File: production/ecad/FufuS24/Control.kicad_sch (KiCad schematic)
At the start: 28 parts, among them IC1 NLVPCA9535EDTR2G, J2 Conn_01x02, U1 RP2040, U2 W25Q128JVS

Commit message: efan 5
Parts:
- J2: footprint (none) -> footprints:CON_5025840270_MOL
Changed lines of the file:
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@@
       (effects (font (size 1.27 1.27)))
     )
-    (property "Footprint" "" (at 20.955 85.09 0)
+    (property "Footprint" "footprints:CON_5025840270_MOL" (at 20.955 85.09 0)
       (effects (font (size 1.27 1.27)) hide)
     )

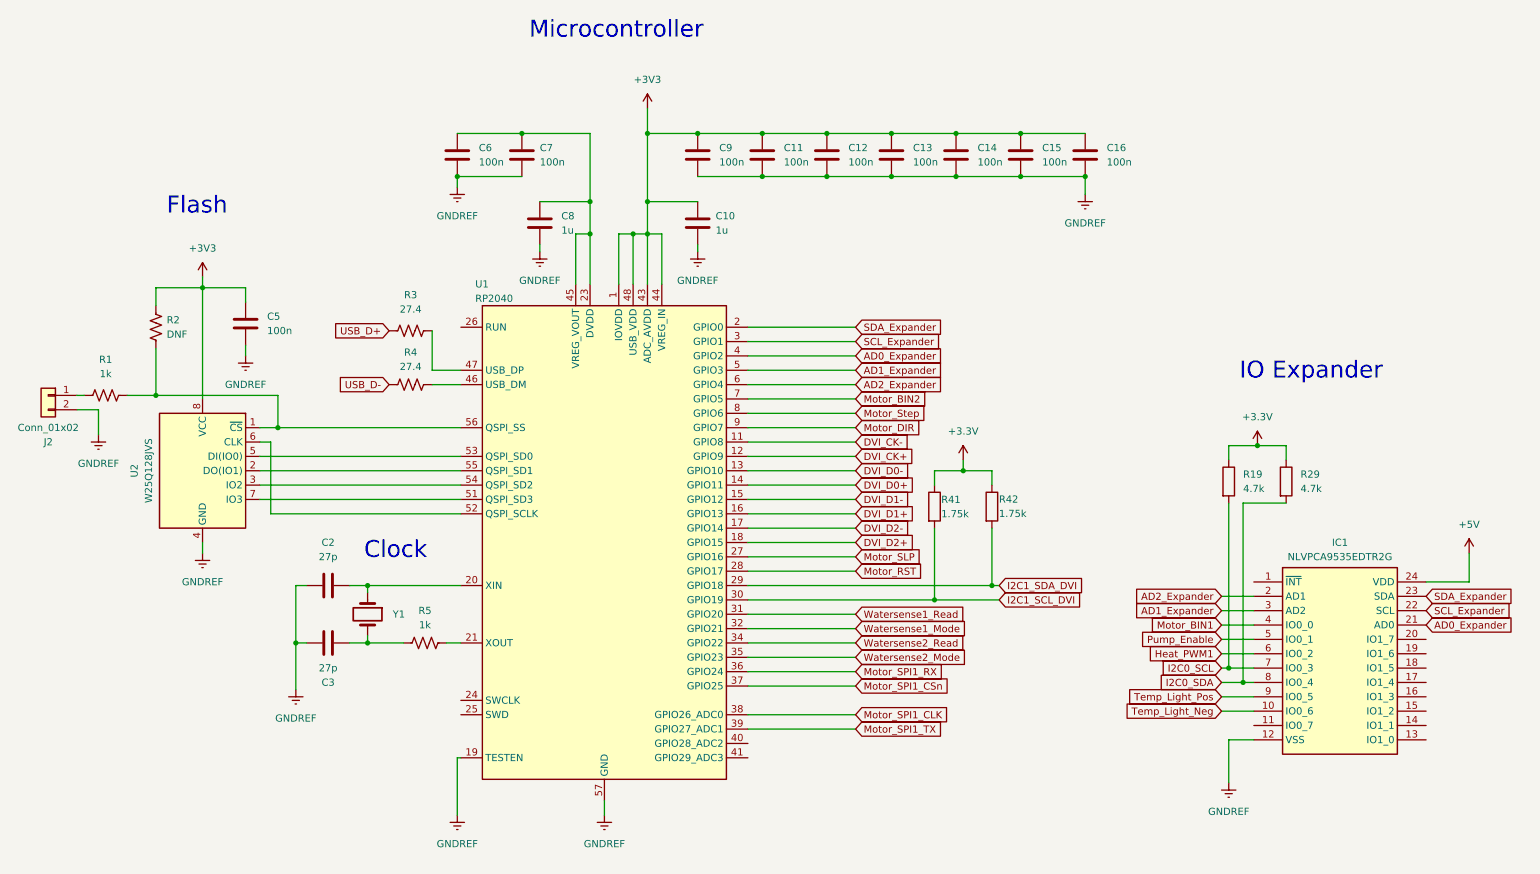
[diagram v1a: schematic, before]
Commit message: goose
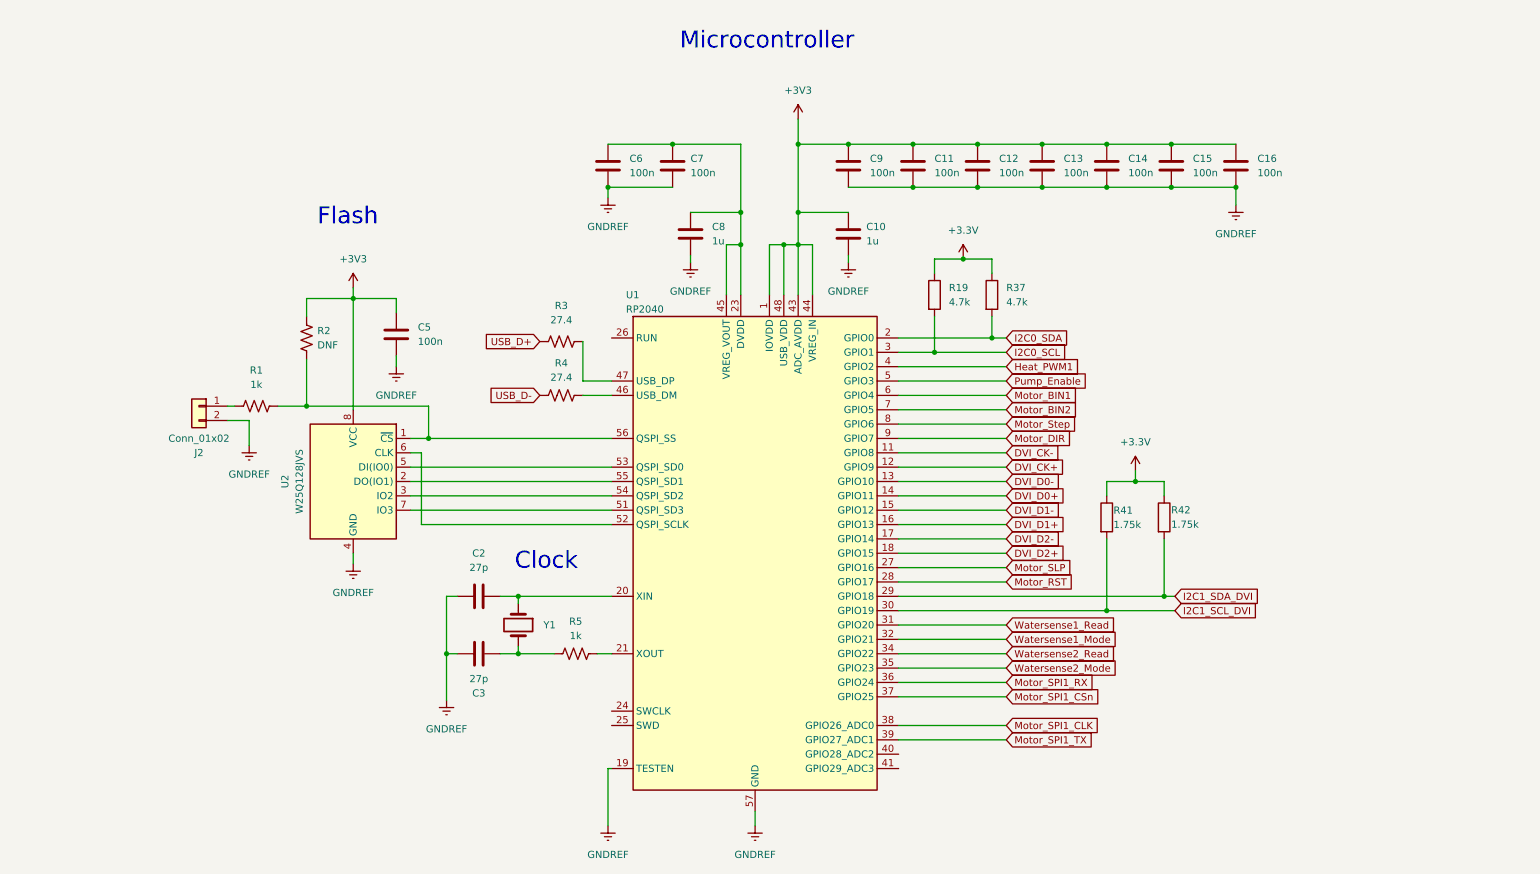
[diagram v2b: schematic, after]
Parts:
- removed IC1: NLVPCA9535EDTR2G, footprints:SOP65P640X120-24N, symbol NLVPCA9535EDTR2G:NLVPCA9535EDTR2G
- removed R29: 4.7k, footprints:RESC2012X60N, symbol Device:R
- added R37: 4.7k, symbol Device:R
- C10, C11, C12, C13, C14, C15, C16, C2, C3, C5, C6, C7, C8, C9: footprint footprints:CAPC2012X94N -> (none)
- J2: footprint footprints:CON_5025840270_MOL -> (none)
- R1, R19, R2, R3, R4, R41, R42, R5: footprint footprints:RESC2012X60N -> (none)
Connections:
- net AD0_Expander is gone; now on net Heat_PWM1: U1.4 (GPIO2)
- net AD1_Expander is gone; now on net Pump_Enable: U1.5 (GPIO3)
- net AD2_Expander is gone; now on net Motor_BIN1: U1.6 (GPIO4)
- net SCL_Expander is gone; now on net I2C0_SCL: U1.3 (GPIO1)
- net SDA_Expander is gone; now on net I2C0_SDA: U1.2 (GPIO0)
- net +3.3V: now also R37.1
- net I2C0_SDA: now also R37.2
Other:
- note removed: "IO Expander"
- moved on the sheet: C10, C11, C12, C13, C14, C15, C16, C2, C3, C5, C6, C7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
